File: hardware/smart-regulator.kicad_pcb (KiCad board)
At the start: 2 copper layers, 82.5 x 48.6 mm, 45 parts, among them J1 Conn_02x05_Odd_Even, P5 USB_A_2, Q1 Q_NMOS_GSD_PSMN038-100YLX, Q2 Q_NMOS_GSD, Q3 Q_PMOS_GSD, U1 ESP-WROOM-32, U10 touchpad, U11 SPX1117M3-L-3-3/TR, U2 Power-Monitor-INA219, U3 LM2576, U4 housing-mounts, U5 Power-Monitor-INA219, U6 SI7020-A20, U7 OPT3001

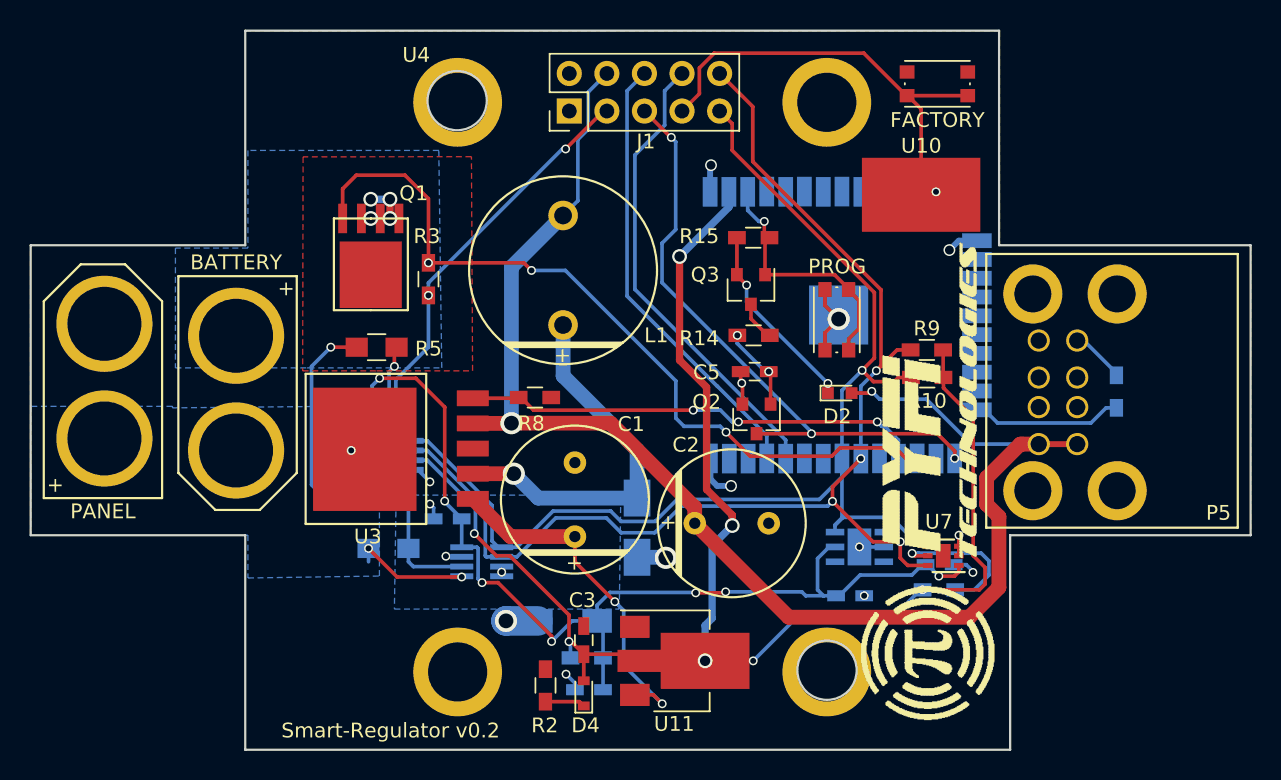
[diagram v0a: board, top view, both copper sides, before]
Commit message: update
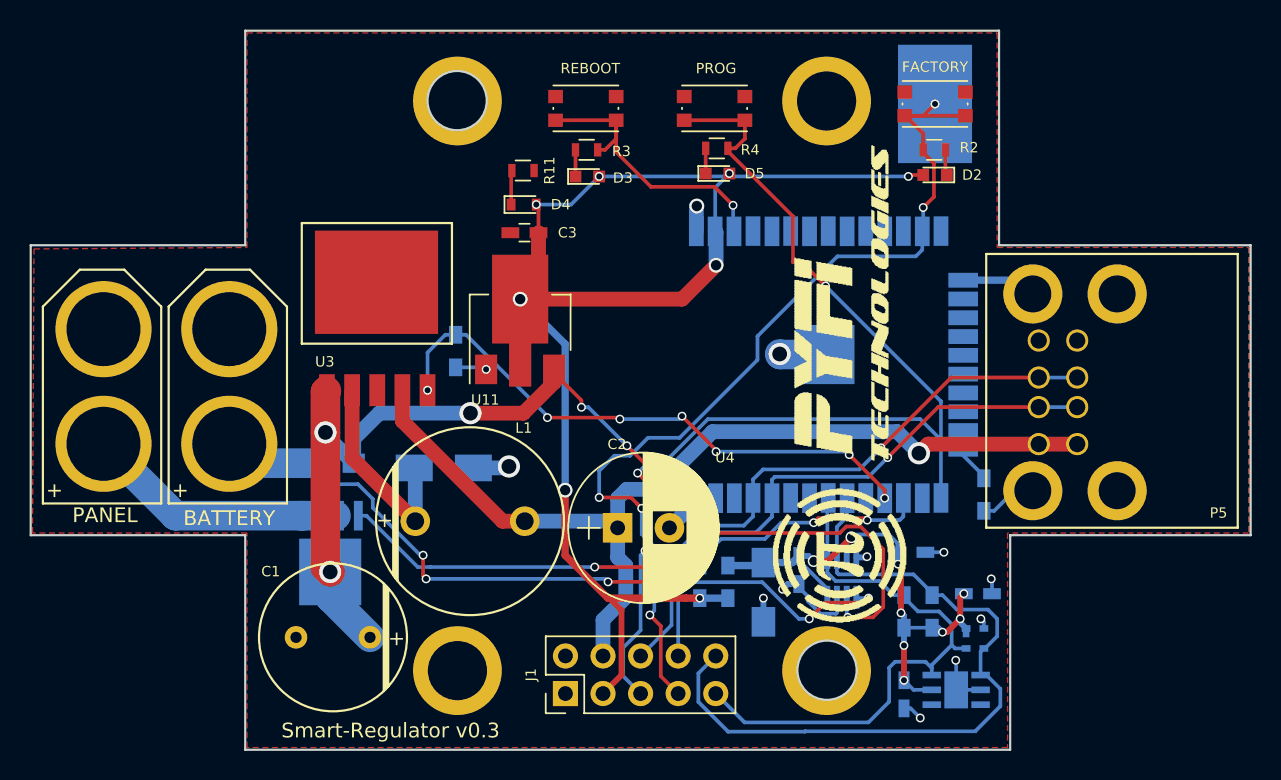
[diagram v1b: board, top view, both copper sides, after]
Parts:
- removed C5: 4.7uF, Capacitors_SMD:C_0603_HandSoldering
- removed C7: C_0.1uF, Capacitors_SMD:C_0603_HandSoldering
- removed Q2: Q_NMOS_GSD, TO_SOT_Packages_SMD:SOT-23
- removed Q3: Q_PMOS_GSD, TO_SOT_Packages_SMD:SOT-23
- removed R14, R15: 1K, Resistors_SMD:R_0603_HandSoldering
- removed U7: OPT3001, Housings_DFN_QFN:DFN-6-1EP_2x2mm_Pitch0.65mm
- added D3: LED, LEDs:LED_0603, F.Cu at (130.8, 87.5)
- added D5: LED, LEDs:LED_0603, F.Cu at (139.6, 87.3)
- added R11: R_10k, Resistors_SMD:R_0603, F.Cu at (126.5, 87.1)
- added REBOOT: SW_PUSH, Buttons_Switches_SMD:SW_SPST_KMR2, F.Cu at (130.7, 82.9)
- C2: footprint open-automation:CAP-RAD-5mm-UVR1H102MHD -> Capacitors_THT:CP_Radial_D10.0mm_P3.50mm
- Q1, R10, R5, R8, R9, U10: moved to B.Cu
- R1: value R_10 -> R_1
- R2, R3: value 1K -> R_10k; footprint Resistors_SMD:R_0603_HandSoldering -> Resistors_SMD:R_0603
- R4: value 50m -> R_10k; footprint Resistors_SMD:R_0805_HandSoldering -> Resistors_SMD:R_0603; moved to F.Cu
- R7: value R_10k -> 1K
- U2: value Power-Monitor-INA219 -> TSL45315CL; footprint TO_SOT_Packages_SMD:SOT-23-8_Handsoldering -> open-automation:LIGHT-SENSOR-TSL45315CL
- U4: footprint footprints:enclosure-25x38 -> open-automation:enclosure-25x38
- moved R2 44.7 mm to (154.3, 85.7), turned to 180 degrees
- moved C8 39.7 mm to (152.7, 112.9), turned to 180 degrees
- moved J1 39.4 mm to (129.4, 122.4)
- moved R4 35.0 mm to (139.6, 85.6)
- moved D4 33.3 mm to (126.5, 89.4), turned to 0 degrees
- moved U2 33.0 mm to (156.4, 118.0), turned to 270 degrees
- moved U5 31.5 mm to (148.0, 114.6), turned to 90 degrees
- moved C3 27.8 mm to (126.6, 91.3), turned to 180 degrees
- moved U11 25.3 mm to (126.3, 97.3), turned to 90 degrees
- moved Q1 20.3 mm to (113.5, 110.4), turned to 0 degrees
- moved C1 18.8 mm to (113.7, 118.6), turned to 180 degrees
- moved L1 18.1 mm to (122.9, 110.8), turned to 0 degrees
- moved R9 17.7 mm to (154.1, 116.9), turned to 270 degrees
- moved PROG 16.5 mm to (139.4, 82.9), turned to 180 degrees
- moved C6 16.3 mm to (145.1, 114.1), turned to 270 degrees
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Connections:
- D2 pad 2: V_USB -> 3V3
- P5 pad 3: Net-(P5-Pad3) -> TXD
- P5 pad 4: Net-(P5-Pad4) -> RXD
- P5 pad 5: Net-(P5-Pad5) -> TXD
- P5 pad 6: Net-(P5-Pad6) -> RXD
- PROG pad 1: EN -> PROG
- Q1 pad 1: BAT_SW -> PANEL_SW
- Q1 pad 2: BATTERY -> V_PANEL
- Q1 pad 3: Net-(Q1-Pad3) -> V_MAIN
- R10 pad 2: 3V3 -> VCC_I2C
- R2 pad 1: Net-(D4-Pad1) -> Net-(D2-Pad1)
- R2 pad 2: GND -> FACTORY
- R3 pad 1: 3V3 -> Net-(D3-Pad1)
- R3 pad 2: BAT_SW -> EN
- R4 pad 1: V_PANEL -> Net-(D5-Pad1)
- R4 pad 2: V_MAIN -> PROG
- R5 pad 1: Net-(Q1-Pad3) -> BATTERY
- R7 pad 1: LIGHT_INT -> 3V3
- R7 pad 2: 3V3 -> PANEL_SW
- R9 pad 2: 3V3 -> VCC_I2C
- U1 pad 27: BAT_SW -> PANEL_SW
- U2 pad 1: V_PANEL -> VCC_I2C
- U2 pad 2: V_MAIN -> GND
- U2 pad 3: GND -> SDA
- U2 pad 4: VCC_I2C -> SCL
- U5 pad 1: Net-(Q1-Pad3) -> BATTERY
- U5 pad 7: 3V3 -> VCC_I2C
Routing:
- net BAT_SW: track 54.2 -> 0.00 mm, vias 4 -> 0
- net BATTERY: track 4.86 -> 51.3 mm, vias 4 -> 6
- net SCL: track 82.7 -> 38.8 mm, vias 2 -> 0
- net PANEL_SW: track 0.00 -> 41.2 mm, vias 0 -> 4
- net VCC_I2C: track 73.1 -> 37.0 mm, vias 7 -> 9
- net 3V3: track 134.8 -> 98.8 mm, vias 9 -> 8
- net PROG: track 41.7 -> 75.8 mm
- net SDA: track 83.6 -> 50.3 mm, vias 4 -> 0
- net FACTORY: track 31.4 -> 64.4 mm, vias 1 -> 5
- net V_USB: track 97.8 -> 65.6 mm, vias 2 -> 1
- net V_MAIN: track 46.3 -> 74.6 mm, vias 3 -> 6
- net Net-(Q1-Pad3): track 16.6 -> 0.00 mm, vias 1 -> 0
- net Net-(D2-Pad1): track 13.1 -> 1.74 mm, vias 2 -> 0
- net Net-(D1-Pad1): track 25.6 -> 14.2 mm, vias 1 -> 0
- net TXD: track 30.4 -> 41.5 mm, vias 0 -> 1
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- removed copper zone on B.Cu, net BATTERY
- removed copper zone on F.Cu, net Net-(Q1-Pad3)
- removed copper zone on B.Cu, net V_MAIN
- removed copper zone on B.Cu, net V_PANEL
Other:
- board text added: "Smart-Regulator v0.3"
- board text removed: "Smart-Regulator v0.2"
